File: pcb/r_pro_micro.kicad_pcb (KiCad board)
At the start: 4 copper layers, 36 x 52 mm, 27 parts, among them J1 Conn_01x12, J2 USB_A, J3 Conn_01x12, U1 MIC5219-2.5YM5, U2 ATmega32U4-MU, Y1 16MHz

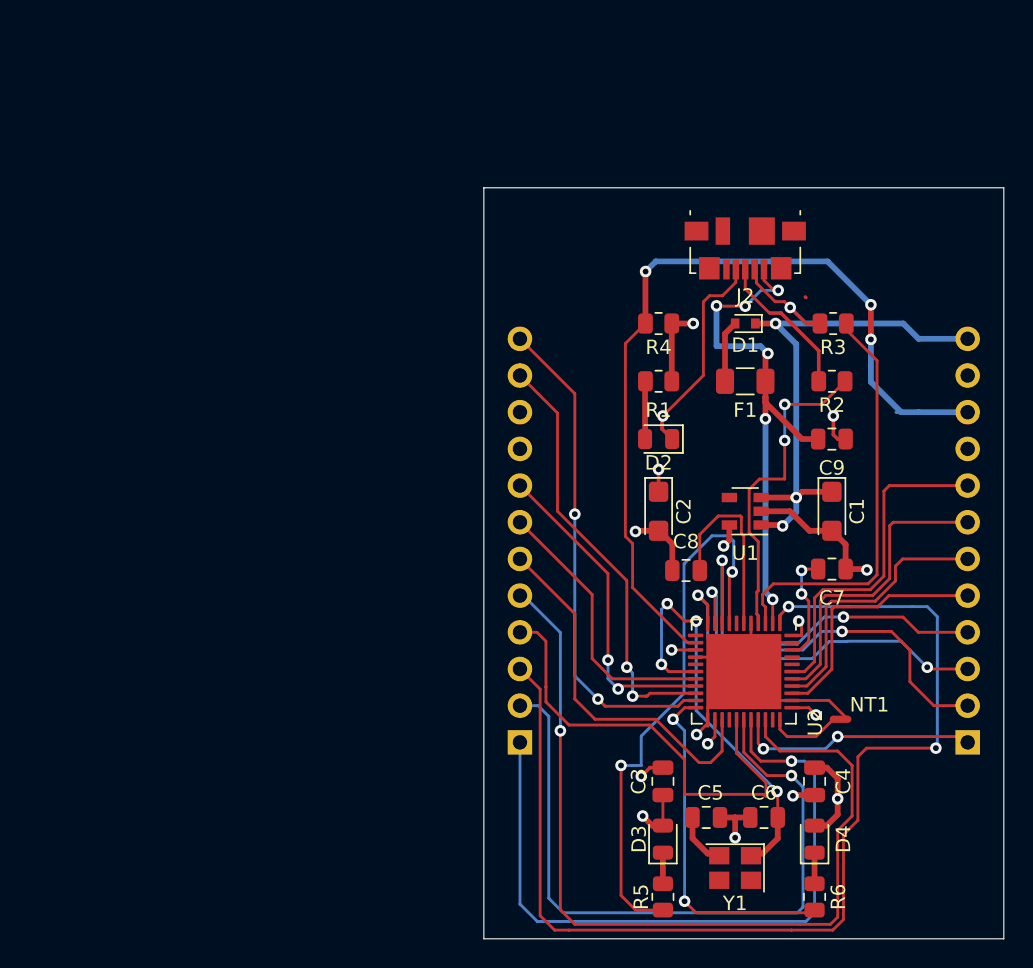
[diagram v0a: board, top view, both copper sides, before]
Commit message: Se reahace PCB
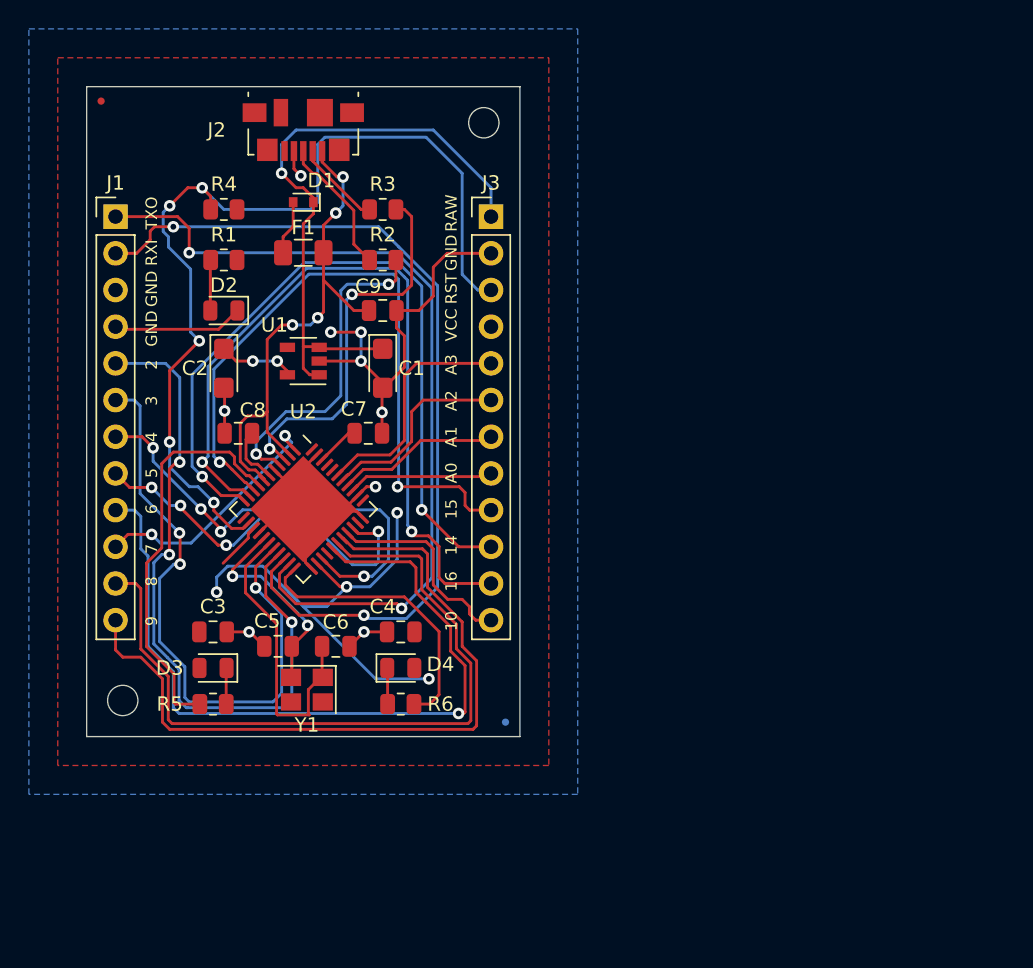
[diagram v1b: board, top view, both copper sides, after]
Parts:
- removed NT1: Net-Tie_2, NetTie:NetTie-2_SMD_Pad0.5mm
- added FID1: Fiducial, Fiducial:Fiducial_0.5mm_Mask1mm, F.Cu at (111.0, 71.0)
- added FID2: Fiducial, Fiducial:Fiducial_0.5mm_Mask1mm, B.Cu at (139.0, 114.0)
- added H1: MountingHole, MountingHole:MountingHole_2.1mm, F.Cu at (137.5, 72.5)
- added H2: MountingHole, MountingHole:MountingHole_2.1mm, F.Cu at (112.5, 112.5)
- J1, J3: moved to F.Cu
- moved J3 49.1 mm to (138.0, 79.0)
- moved J1 45.9 mm to (112.0, 79.0)
- moved R5 33.9 mm to (118.8, 112.8), turned to 180 degrees
- moved C7 33.4 mm to (129.5, 94.0)
- moved D3 33.3 mm to (118.8, 110.2), turned to 180 degrees
- moved C3 32.8 mm to (118.8, 107.8), turned to 0 degrees
- moved C1 32.6 mm to (130.5, 89.5)
- moved U2 32.5 mm to (125.0, 99.2), turned to 315 degrees
- moved C8 32.4 mm to (120.5, 94.0)
- moved C9 32.3 mm to (130.5, 85.5)
- moved U1 32.3 mm to (125.0, 89.0)
- moved R2 32.2 mm to (130.5, 82.0)
- moved R3 32.2 mm to (130.5, 78.5)
- moved Y1 32.1 mm to (125.2, 111.8)
- moved C5 31.9 mm to (123.2, 108.8), turned to 180 degrees
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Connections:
- J1 pad 1: /D9 -> /TXO
- J1 pad 10: GND -> /D7
- J1 pad 11: /RXI -> /D8
- J1 pad 12: /TXO -> /D9
- J1 pad 2: /D8 -> /RXI
- J1 pad 3: /D7 -> GND
- J1 pad 4: /D6 -> GND
- J1 pad 5: /D5 -> /D2
- J1 pad 6: /D4 -> /D3
- J1 pad 7: /D3 -> /D4
- J1 pad 8: /D2 -> /D5
- J1 pad 9: GND -> /D6
- J3 pad 1: /D10 -> /RAW
- J3 pad 10: /RESET -> /MISO
- J3 pad 11: GND -> /MOSI
- J3 pad 12: /RAW -> /D10
- J3 pad 2: /MOSI -> GND
- J3 pad 3: /MISO -> /RESET
- J3 pad 4: /SCK -> +3V3
- J3 pad 5: /A0 -> /A3
- J3 pad 6: /A1 -> /A2
- J3 pad 7: /A2 -> /A1
- J3 pad 8: /A3 -> /A0
- J3 pad 9: +3V3 -> /SCK
- U2 pad 33: Net-(NT1-Pad1) -> GND
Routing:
- net /D7: track 77.8 -> 18.0 mm
- net /D5: track 62.5 -> 27.4 mm, vias 1 -> 4
- net /RXI: track 29.9 -> 61.7 mm
- net /MISO: track 25.3 -> 52.0 mm
- net /MOSI: track 27.2 -> 53.8 mm
- net /D2: track 22.3 -> 48.7 mm, vias 2 -> 3
- net /TXO: track 34.3 -> 59.0 mm
- net /D3: track 19.3 -> 43.2 mm, vias 0 -> 3
- net /D6: track 31.8 -> 54.3 mm, vias 0 -> 1
- net /SCK: track 28.0 -> 47.5 mm
- net +3V3: track 25.9 -> 42.9 mm, vias 9 -> 6
- net GND: track 64.2 -> 77.5 mm, vias 8 -> 9
- net Net-(R5-Pad2): track 39.1 -> 27.9 mm, vias 2 -> 0
- net Net-(C5-Pad1): track 3.33 -> 14.3 mm, vias 0 -> 2
- net Net-(C8-Pad1): track 13.4 -> 4.01 mm
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- added copper zone on F.Cu, net +3V3
- added copper zone on B.Cu, net GND
- removed copper zone on In2.Cu.3V3, net +3V3
- removed copper zone on In1.Cu.GND, net GND
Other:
- board size 36 x 52 mm -> 30 x 45 mm
- copper layers 4 -> 2
- board text added: "10"
- board text added: "14"
- board text added: "15"
- board text added: "16"
- board text added: "2"
- board text added: "3"
- board text added: "4"
- board text added: "5"
- board text added: "6"
- board text added: "7"
- board text added: "8"
- board text added: "9"
- board text added: "A0"
- board text added: "A1"
- board text added: "A2"
- board text added: "A3"
- board text added: "GND"
- board text added: "RAW"
- board text added: "RST"
- board text added: "RXI"
- board text added: "TXO"
- board text added: "VCC"
